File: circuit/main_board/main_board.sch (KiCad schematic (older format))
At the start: 19 parts

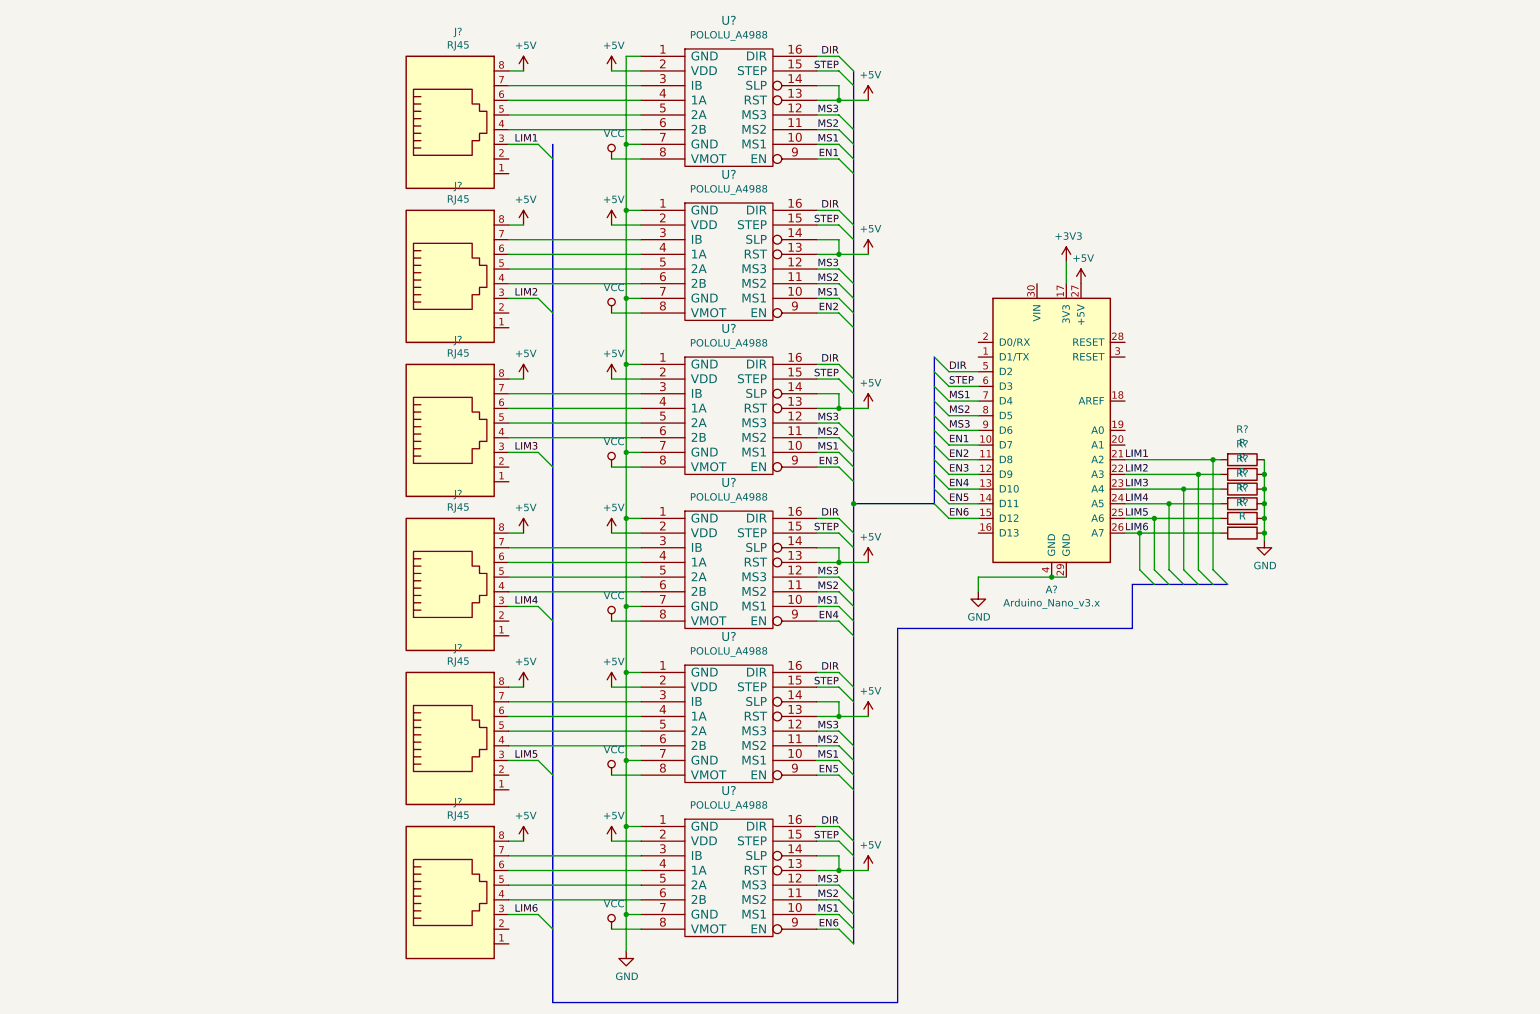
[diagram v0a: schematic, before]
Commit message: Second revision
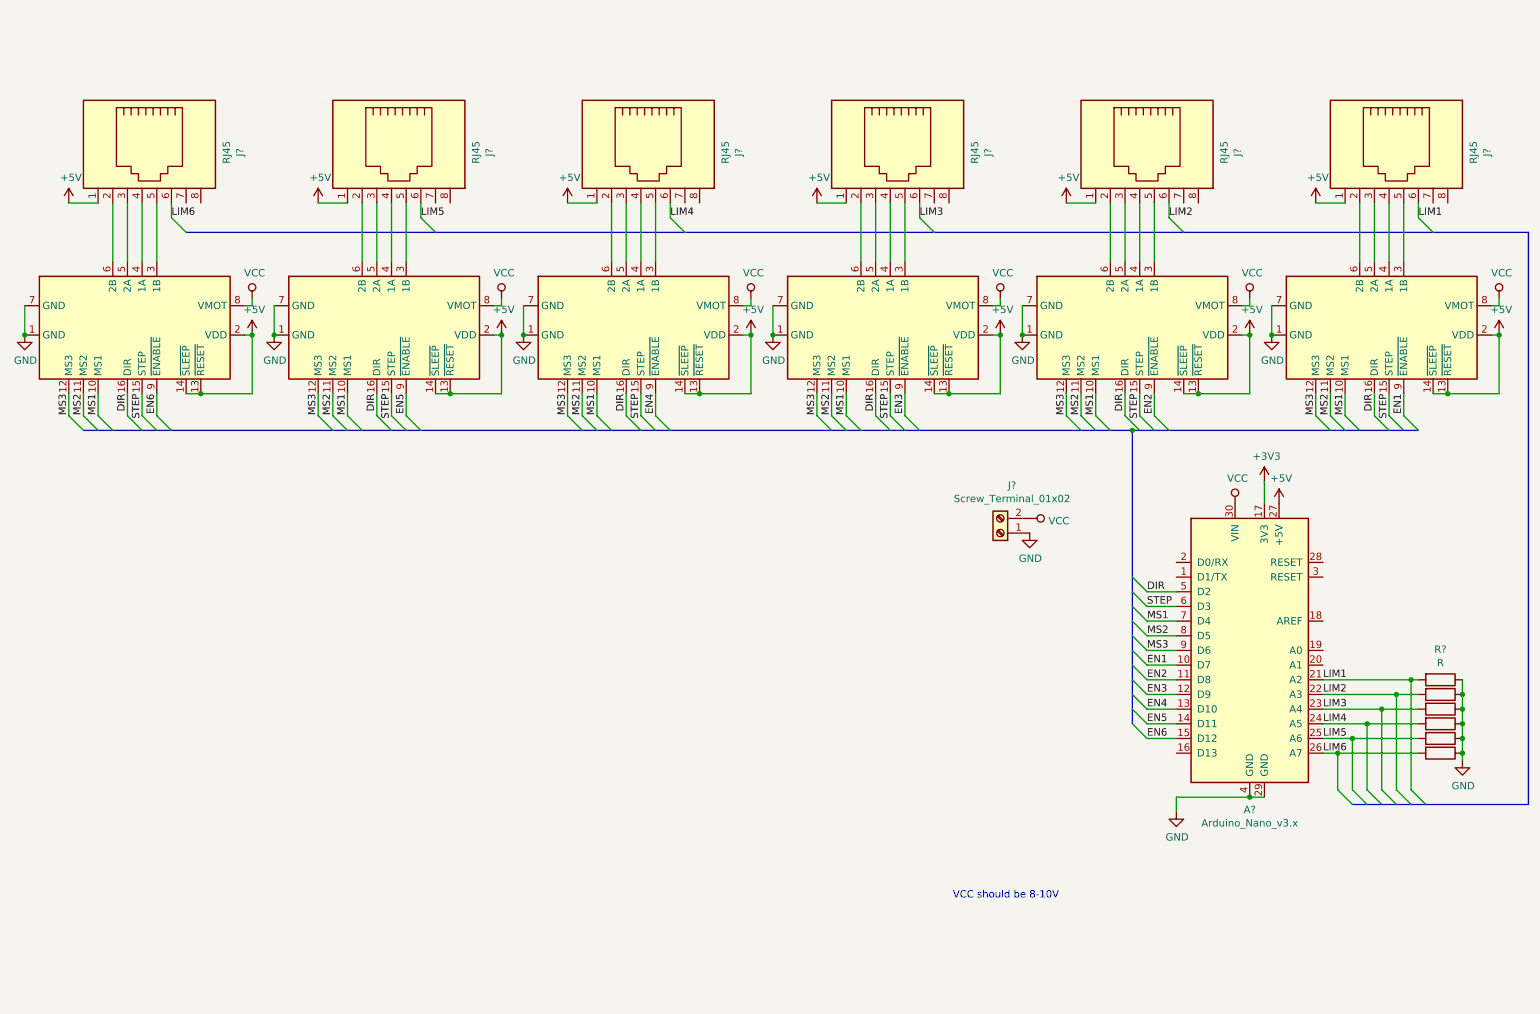
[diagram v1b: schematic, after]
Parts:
- removed J? (x5): RJ45, symbol Connector:RJ45
- removed R? (x5): R, symbol Device:R
- removed U? (x6): POLOLU_A4988, symbol pololu_a4988:POLOLU_A4988
- added A? (x6): Pololu_Breakout_A4988, Module:Pololu_Breakout-16_15.2x20.3mm, symbol Driver_Motor:Pololu_Breakout_A4988
- added J? (x5): RJ45, Connector_RJ:RJ45_Wuerth_7499010121A_Horizontal, symbol Connector:RJ45
- added J?: Screw_Terminal_01x02, TerminalBlock:TerminalBlock_Altech_AK300-2_P5.00mm, symbol Connector:Screw_Terminal_01x02
- added R? (x5): R, Resistor_THT:R_Axial_DIN0309_L9.0mm_D3.2mm_P15.24mm_Horizontal, symbol Device:R
- J?: footprint (none) -> Connector_RJ:RJ45_Wuerth_7499010121A_Horizontal
- R?: footprint (none) -> Resistor_THT:R_Axial_DIN0309_L9.0mm_D3.2mm_P15.24mm_Horizontal
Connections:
- net +5V: now also J?.1, A?.13 (~RESET), A?.13 (~RESET), A?.13 (~RESET), A?.13 (~RESET), A?.13 (~RESET), A?.13 (~RESET), A?.14 (~SLEEP), A?.14 (~SLEEP), A?.14 (~SLEEP), A?.14 (~SLEEP), A?.14 (~SLEEP), A?.14 (~SLEEP), A?.2 (VDD), A?.2 (VDD), A?.2 (VDD), A?.2 (VDD), A?.2 (VDD), A?.2 (VDD), J?.1, J?.1, J?.1, J?.1, J?.1; no longer J?.8
- net DIR: now also A?.16 (DIR), A?.16 (DIR), A?.16 (DIR), A?.16 (DIR), A?.16 (DIR), A?.16 (DIR)
- net EN1: now also A?.9 (~ENABLE)
- net EN2: now also A?.9 (~ENABLE)
- net EN3: now also A?.9 (~ENABLE)
- net EN4: now also A?.9 (~ENABLE)
- net EN5: now also A?.9 (~ENABLE)
- net EN6: now also A?.9 (~ENABLE)
- net GND: now also A?.1 (GND), A?.1 (GND), A?.1 (GND), A?.1 (GND), A?.1 (GND), A?.1 (GND), A?.7 (GND), A?.7 (GND), A?.7 (GND), A?.7 (GND), A?.7 (GND), A?.7 (GND), J?.1 (Pin_1), R?.1, R?.1, R?.1, R?.1, R?.1
- net LIM1: now also J?.6, R?.2
- net LIM2: now also J?.6, R?.2
- net LIM3: now also J?.6, R?.2
- net LIM4: now also J?.6, R?.2
- net LIM5: now also J?.6, R?.2
- net LIM6: now also J?.6; no longer J?.3
- net MS1: now also A?.10 (MS1), A?.10 (MS1), A?.10 (MS1), A?.10 (MS1), A?.10 (MS1), A?.10 (MS1)
- net MS2: now also A?.11 (MS2), A?.11 (MS2), A?.11 (MS2), A?.11 (MS2), A?.11 (MS2), A?.11 (MS2)
- net MS3: now also A?.12 (MS3), A?.12 (MS3), A?.12 (MS3), A?.12 (MS3), A?.12 (MS3), A?.12 (MS3)
- net STEP: now also A?.15 (STEP), A?.15 (STEP), A?.15 (STEP), A?.15 (STEP), A?.15 (STEP), A?.15 (STEP)
- net VCC: now also A?.30 (VIN), A?.8 (VMOT), A?.8 (VMOT), A?.8 (VMOT), A?.8 (VMOT), A?.8 (VMOT), A?.8 (VMOT), J?.2 (Pin_2)
- net at J?.5: now also A?.3 (1B)
- net at J?.4: now also A?.4 (1A)
- net at J?.2: now also A?.6 (2B)
- new net: A?.3 (1B), J?.5 (x5)
- new net: A?.4 (1A), J?.4 (x5)
- new net: A?.5 (2A), J?.3 (x6)
- new net: A?.6 (2B), J?.2 (x5)
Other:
- note added: "VCC should be 8-10V"
- moved on the sheet: A?, J?
